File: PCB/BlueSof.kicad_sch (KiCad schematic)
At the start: 109 parts, among them J1 USB_C_Receptacle_USB2.0, J2 Conn_01x01_Female, J3 Conn_01x04_Female, J4 Conn_01x01_Female, J5 USB_C_Receptacle_USB2.0, Q1 A03407, Q2 A03407, SW1 SW_PUSH, SW10 SW_PUSH, SW11 SW_PUSH, SW12 SW_PUSH, SW13 SW_PUSH, SW14 SW_PUSH, SW15 SW_PUSH, SW16 SW_PUSH, SW17 SW_PUSH, SW18 SW_PUSH, SW19 SW_PUSH, SW2 SW_PUSH, SW20 SW_PUSH, SW21 SW_PUSH, SW22 SW_PUSH, SW23 SW_PUSH, SW24 SW_PUSH, SW25 Rotary_Encoder_Switch, SW26 SW_PUSH, SW27 SW_PUSH, SW28 SW_PUSH, SW29 SW_PUSH, SW3 SW_PUSH, SW30 SW_PUSH, SW31 SW_Push, SW32 SW_Push, SW4 SW_PUSH, SW5 SW_PUSH, SW6 SW_PUSH, SW7 SW_PUSH, SW8 SW_PUSH, SW9 SW_PUSH, U1 LN2054Y42AMR, U2 E73-2G4M08S1C, U3 AP2112K-3.3, U4 E73-2G4M08S1C, U5 LN2054Y42AMR, U6 AP2112K-3.3, Y1 32.768kHz, Y2 32.768kHz

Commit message: first commit, side 1
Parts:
- removed C10: 10uF, Capacitor_SMD:C_0603_1608Metric_Pad1.08x0.95mm_HandSolder, symbol Device:C_Small
- removed C6, C7: 22pF, Capacitor_SMD:C_0603_1608Metric_Pad1.08x0.95mm_HandSolder, symbol Device:C_Small
- removed C8, C9: 4.7uF, Capacitor_SMD:C_0603_1608Metric_Pad1.08x0.95mm_HandSolder, symbol Device:C_Small
- removed D29, D30: D, BlueSof:Diode_SOD123, symbol BlueSof-rescue:D-Lily58-cache-Lily58_Pro-rescue-SofleKeyboard-rescue
- removed D34, D36: LED, LED_SMD:LED_0603_1608Metric_Pad1.05x0.95mm_HandSolder, symbol Device:LED
- removed D35: 1N5819, Diode_SMD:D_SOD-323_HandSoldering, symbol Diode:1N5819
- removed J5: USB_C_Receptacle_USB2.0, Connector_USB:USB_C_Receptacle_HRO_TYPE-C-31-M-12, symbol Connector:USB_C_Receptacle_USB2.0
- removed Q1: A03407, Package_TO_SOT_SMD:SOT-23, symbol Device:Q_PMOS_GSD
- removed R10: 2M, Resistor_SMD:R_0603_1608Metric_Pad0.98x0.95mm_HandSolder, symbol Device:R_Small
- removed R11, R15: 1k, Resistor_SMD:R_0603_1608Metric_Pad0.98x0.95mm_HandSolder, symbol Device:R_Small
- removed R12, R13: 5.1k, Resistor_SMD:R_0603_1608Metric_Pad0.98x0.95mm_HandSolder, symbol Device:R_Small
- removed R14: 100k, Resistor_SMD:R_0603_1608Metric_Pad0.98x0.95mm_HandSolder, symbol Device:R_Small
- removed R16: 10k, Resistor_SMD:R_0603_1608Metric_Pad0.98x0.95mm_HandSolder, symbol Device:R_Small
- removed R3: 820k, Resistor_SMD:R_0603_1608Metric_Pad0.98x0.95mm_HandSolder, symbol Device:R_Small
- removed SW29, SW30: SW_PUSH, BlueSof:KailhLowProfile, symbol BlueSof-rescue:SW_PUSH-Lily58-cache-Lily58_Pro-rescue-SofleKeyboard-rescue
- removed SW32: SW_Push, Button_Switch_SMD:SW_SPST_B3U-1000P, symbol Switch:SW_Push
- removed U4: E73-2G4M08S1C, BlueSof:E73-2G4M08S1C-52840, symbol BlueSof-rescue:E73-2G4M08S1C-ELLOW
- removed U5: LN2054Y42AMR, Package_TO_SOT_SMD:SOT-23-5, symbol BlueSof-rescue:LN2054Y42AMR-ELLOW
- removed U6: AP2112K-3.3, Package_TO_SOT_SMD:SOT-23-5, symbol Regulator_Linear:AP2112K-3.3
- removed Y2: 32.768kHz, Crystal:Crystal_SMD_MicroCrystal_CM9V-T1A-2Pin_1.6x1.0mm_HandSoldering, symbol Device:Crystal
- added J9: Conn_01x04_Female, Connector_PinHeader_2.54mm:PinHeader_1x04_P2.54mm_Vertical, symbol Connector:Conn_01x04_Female
- added SW59: SW_SPDT, Button_Switch_THT:SW_CuK_OS102011MA1QN1_SPDT_Angled, symbol Switch:SW_SPDT
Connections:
- net DATA+: now also J9.3 (Pin_3)
- net DATA-: now also J9.4 (Pin_4)
- net ENCA: now also U2.33 (P0.13); no longer U2.10 (P0.30/AIN6)
- net ENCB: now also U2.35 (P0.24); no longer U2.9 (P0.31/AIN7)
- net GND: now also J9.1 (Pin_1)
- net VBAT: now also SW59.1 (A); no longer Q2.3 (D)
- net VBUS: now also J9.2 (Pin_2)
- net row1: now also U2.10 (P0.30/AIN6); no longer U2.33 (P0.13)
- net row2: now also U2.9 (P0.31/AIN7); no longer U2.35 (P0.24)
- new net: Q2.3 (D), SW59.2 (B)
- no-connect marks 32 -> 16
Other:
- note added: "USB Header"
- note removed: "Left Side"
- moved on the sheet: C1, C2, C3, C4, C5, D1, D10, D11, D12, D13, D14, D15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

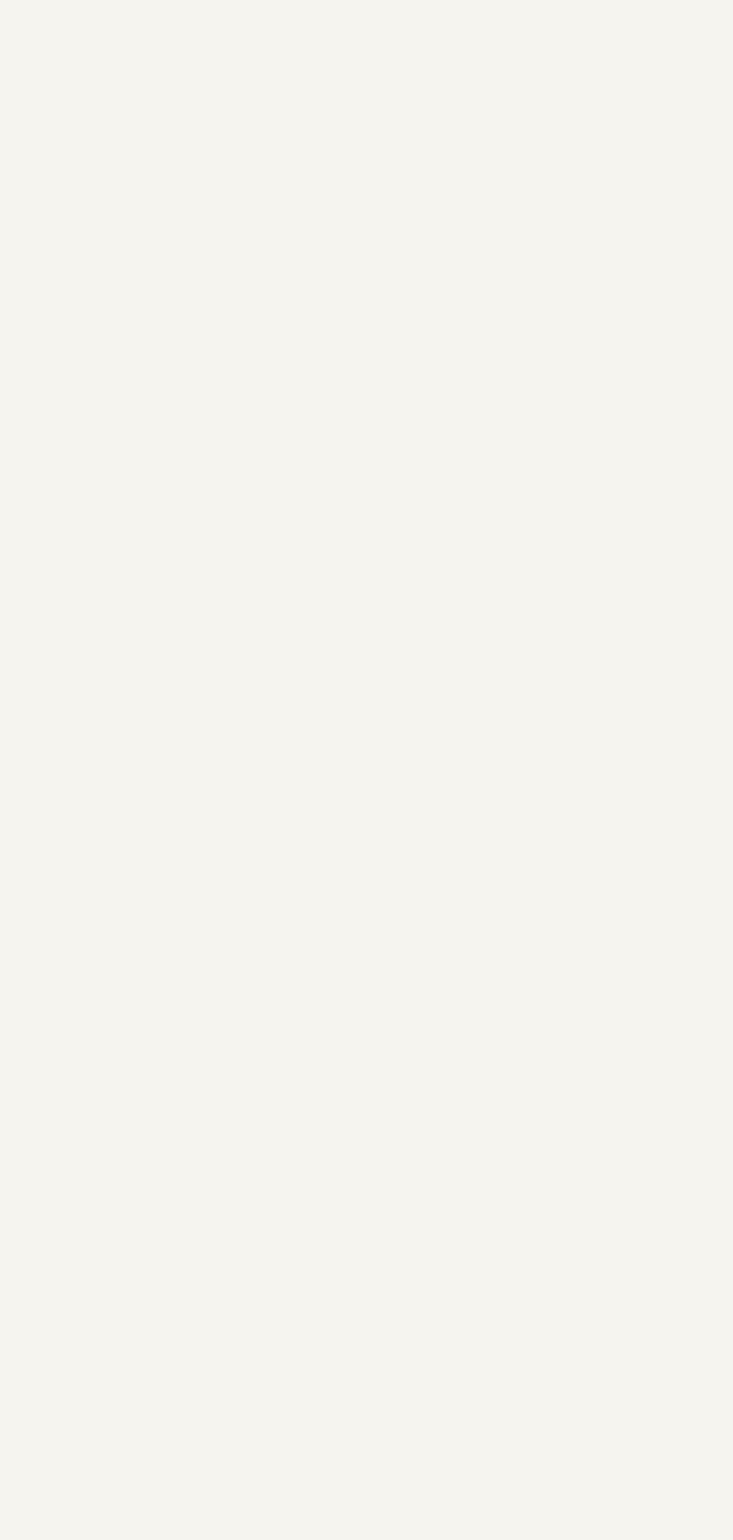
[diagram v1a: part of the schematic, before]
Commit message: EOD
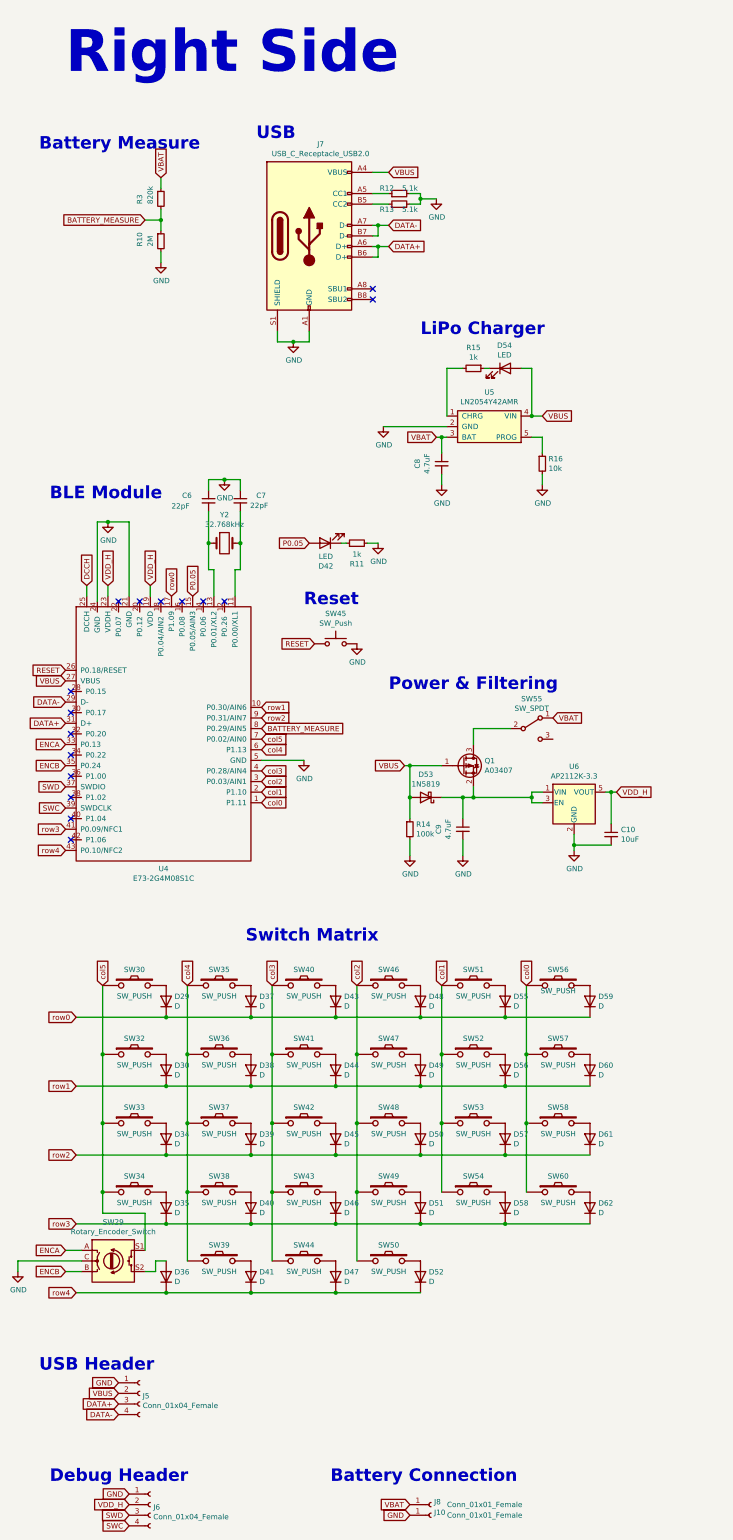
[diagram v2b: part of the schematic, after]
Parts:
- added C10: 10uF, Capacitor_SMD:C_0603_1608Metric_Pad1.08x0.95mm_HandSolder, symbol Device:C_Small
- added C6, C7: 22pF, Capacitor_SMD:C_0603_1608Metric_Pad1.08x0.95mm_HandSolder, symbol Device:C_Small
- added C8, C9: 4.7uF, Capacitor_SMD:C_0603_1608Metric_Pad1.08x0.95mm_HandSolder, symbol Device:C_Small
- added D29, D30, D34, D35, D36, D37, D38, D39, D40, D41, D43, D44, D45, D46, D47, D48, D49, D50, D51, D52, D55, D56, D57, D58, D59, D60, D61, D62: D, BlueSof:Diode_SOD123, symbol BlueSof-rescue:D-Lily58-cache-Lily58_Pro-rescue-SofleKeyboard-rescue
- added D42, D54: LED, LED_SMD:LED_0603_1608Metric_Pad1.05x0.95mm_HandSolder, symbol Device:LED
- added D53: 1N5819, Diode_SMD:D_SOD-323_HandSoldering, symbol Diode:1N5819
- added J10, J8: Conn_01x01_Female, Connector_PinHeader_2.54mm:PinHeader_1x01_P2.54mm_Vertical, symbol Connector:Conn_01x01_Female
- added J5, J6: Conn_01x04_Female, Connector_PinHeader_2.54mm:PinHeader_1x04_P2.54mm_Vertical, symbol Connector:Conn_01x04_Female
- added J7: USB_C_Receptacle_USB2.0, BlueSof:USB-C_C168688, symbol Connector:USB_C_Receptacle_USB2.0
- added Q1: A03407, Package_TO_SOT_SMD:SOT-23, symbol Device:Q_PMOS_GSD
- added R10: 2M, Resistor_SMD:R_0603_1608Metric_Pad0.98x0.95mm_HandSolder, symbol Device:R_Small
- added R11, R15: 1k, Resistor_SMD:R_0603_1608Metric_Pad0.98x0.95mm_HandSolder, symbol Device:R_Small
- added R12, R13: 5.1k, Resistor_SMD:R_0603_1608Metric_Pad0.98x0.95mm_HandSolder, symbol Device:R_Small
- added R14: 100k, Resistor_SMD:R_0603_1608Metric_Pad0.98x0.95mm_HandSolder, symbol Device:R_Small
- added R16: 10k, Resistor_SMD:R_0603_1608Metric_Pad0.98x0.95mm_HandSolder, symbol Device:R_Small
- added R3: 820k, Resistor_SMD:R_0603_1608Metric_Pad0.98x0.95mm_HandSolder, symbol Device:R_Small
- added SW29: Rotary_Encoder_Switch, Rotary_Encoder:RotaryEncoder_Alps_EC11E-Switch_Vertical_H20mm, symbol BlueSof-rescue:Rotary_Encoder_Switch-Device-SofleKeyboard-rescue
- added SW30, SW32, SW33, SW34, SW35, SW36, SW37, SW38, SW40, SW41, SW42, SW43, SW44, SW46, SW47, SW48, SW49, SW50, SW51, SW52, SW53, SW54, SW56, SW57, SW58, SW60: SW_PUSH, BlueSof:KailhLowProfile, symbol BlueSof-rescue:SW_PUSH-Lily58-cache-Lily58_Pro-rescue-SofleKeyboard-rescue
- added SW39: SW_PUSH, BlueSof:KailhLowProfile_1.5U, symbol BlueSof-rescue:SW_PUSH-Lily58-cache-Lily58_Pro-rescue-SofleKeyboard-rescue
- added SW45: SW_Push, Button_Switch_SMD:SW_SPST_B3U-1000P, symbol Switch:SW_Push
- added SW55: SW_SPDT, Button_Switch_THT:SW_CuK_OS102011MA1QN1_SPDT_Angled, symbol Switch:SW_SPDT
- added U4: E73-2G4M08S1C, BlueSof:E73-2G4M08S1C-52840, symbol BlueSof-rescue:E73-2G4M08S1C-ELLOW
- added U5: LN2054Y42AMR, Package_TO_SOT_SMD:SOT-23-5, symbol BlueSof-rescue:LN2054Y42AMR-ELLOW
- added U6: AP2112K-3.3, Package_TO_SOT_SMD:SOT-23-5, symbol Regulator_Linear:AP2112K-3.3
- added Y2: 32.768kHz, Crystal:Crystal_SMD_MicroCrystal_CM9V-T1A-2Pin_1.6x1.0mm_HandSoldering, symbol Device:Crystal
- J1: footprint Connector_USB:USB_C_Receptacle_HRO_TYPE-C-31-M-12 -> BlueSof:USB-C_C168688
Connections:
- net BATTERY_MEASURE: now also R10.1, R3.2, U4.8 (P0.29/AIN5)
- net DATA+: now also J5.3 (Pin_3), J7.A6 (D+), J7.B6 (D+), U4.31 (D+)
- net DATA-: now also J5.4 (Pin_4), J7.A7 (D-), J7.B7 (D-), U4.29 (D-)
- net DCCH: now also U4.25 (DCCH)
- net ENCA: now also SW29.A, U4.33 (P0.13)
- net ENCB: now also SW29.B, U4.35 (P0.24)
- net GND: now also C10.2, C6.1, C7.1, C8.2, C9.2, J10.1 (Pin_1), J5.1 (Pin_1), J6.1 (Pin_1), J7.A1 (GND), J7.A12 (GND), J7.B1 (GND), J7.B12 (GND), J7.S1 (SHIELD), R10.2, R11.2, R12.2, R13.2, R14.2, R16.2, SW29.C, SW45.2, U4.21 (GND), U4.24 (GND), U4.5 (GND), U5.2 (GND), U6.2 (GND)
- net P0.05: now also D42.2 (A), U4.15 (P0.05/AIN3)
- net RESET: now also SW45.1, U4.26 (P0.18/RESET)
- net SWC: now also J6.4 (Pin_4), U4.39 (SWDCLK)
- net SWD: now also J6.3 (Pin_3), U4.37 (SWDIO)
- net VBAT: now also C8.1, J8.1 (Pin_1), R3.1, SW55.1 (A), U5.3 (BAT)
- net VBUS: now also D53.2 (A), D54.2 (A), J5.2 (Pin_2), J7.A4 (VBUS), J7.A9 (VBUS), J7.B4 (VBUS), J7.B9 (VBUS), Q1.1 (G), R14.1, U4.27 (VBUS), U5.4 (VIN)
- net VDD_H: now also C10.1, J6.2 (Pin_2), U4.19 (VDD), U4.23 (VDDH), U6.5 (VOUT)
- net col0: now also SW56.1, SW57.1, SW58.1, SW60.1, U4.1 (P1.11)
- net col1: now also SW51.1, SW52.1, SW53.1, SW54.1, U4.2 (P1.10)
- net col2: now also SW46.1, SW47.1, SW48.1, SW49.1, SW50.1, U4.3 (P0.03/AIN1)
- net col3: now also SW40.1, SW41.1, SW42.1, SW43.1, SW44.1, U4.4 (P0.28/AIN4)
- net col4: now also SW35.1, SW36.1, SW37.1, SW38.1, SW39.1, U4.6 (P1.13)
- net col5: now also SW29.S1, SW30.1, SW32.1, SW33.1, SW34.1, U4.7 (P0.02/AIN0)
- net row0: now also D29.1 (K), D37.1 (K), D43.1 (K), D48.1 (K), D55.1 (K), D59.1 (K), U4.17 (P1.09)
- net row1: now also D30.1 (K), D38.1 (K), D44.1 (K), D49.1 (K), D56.1 (K), D60.1 (K), U4.10 (P0.30/AIN6)
- net row2: now also D34.1 (K), D39.1 (K), D45.1 (K), D50.1 (K), D57.1 (K), D61.1 (K), U4.9 (P0.31/AIN7)
- net row3: now also D35.1 (K), D40.1 (K), D46.1 (K), D51.1 (K), D58.1 (K), D62.1 (K), U4.41 (P0.09/NFC1)
- net row4: now also D36.1 (K), D41.1 (K), D47.1 (K), D52.1 (K), U4.43 (P0.10/NFC2)
- new net: J7.A5 (CC1), R12.1
- new net: J7.B5 (CC2), R13.1
- new net: D54.1 (K), R15.1
- new net: R15.2, U5.1 (CHRG)
- new net: D60.2 (A), SW57.2
- new net: D40.2 (A), SW38.2
- new net: D52.2 (A), SW50.2
- new net: D62.2 (A), SW60.2
- new net: C7.2, U4.11 (P0.00/XL1), Y2.2
- new net: C6.2, U4.13 (P0.01/XL2), Y2.1
- new net: D44.2 (A), SW41.2
- new net: D56.2 (A), SW52.2
- new net: D29.2 (A), SW30.2
- new net: D39.2 (A), SW37.2
- new net: D46.2 (A), SW43.2
- new net: Q1.3 (D), SW55.2 (B)
- new net: D34.2 (A), SW33.2
- new net: D48.2 (A), SW46.2
- new net: D49.2 (A), SW47.2
- new net: D37.2 (A), SW35.2
- new net: D61.2 (A), SW58.2
- new net: D30.2 (A), SW32.2
- new net: D45.2 (A), SW42.2
- new net: D41.2 (A), SW39.2
- new net: D36.2 (A), SW29.S2
- new net: D47.2 (A), SW44.2
- new net: D57.2 (A), SW53.2
- new net: C9.1, D53.1 (K), Q1.2 (S), U6.1 (VIN), U6.3 (EN)
- new net: D55.2 (A), SW51.2
- new net: D59.2 (A), SW56.2
- new net: D35.2 (A), SW34.2
- new net: R16.1, U5.5 (PROG)
- new net: D51.2 (A), SW49.2
- new net: D42.1 (K), R11.1
- new net: D50.2 (A), SW48.2
- new net: D43.2 (A), SW40.2
- new net: D58.2 (A), SW54.2
- new net: D38.2 (A), SW36.2
- no-connect marks 16 -> 32

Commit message: getting close to layout on side 1
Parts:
- D1, D10, D11, D12, D13, D14, D15, D16, D17, D18, D19, D2, D20, D21, D22, D23, D24, D25, D26, D27, D28, D29, D3, D30, D34, D35, D36, D37, D38, D39, D4, D40, D41, D43, D44, D45, D46, D47, D48, D49, D5, D50, D51, D52, D55, D56, D57, D58, D59, D6, D60, D61, D62, D7, D8, D9: footprint BlueSof:Diode_SOD123 -> Diode_SMD:D_SOD-123; symbol BlueSof-rescue:D-Lily58-cache-Lily58_Pro-rescue-SofleKeyboard-rescue -> Diode:1N4148
- SW1, SW10, SW11, SW12, SW13, SW14, SW15, SW16, SW17, SW18, SW19, SW2, SW20, SW21, SW22, SW23, SW24, SW26, SW27, SW28, SW3, SW30, SW32, SW33, SW34, SW35, SW36, SW37, SW38, SW39, SW4, SW40, SW41, SW42, SW43, SW44, SW46, SW47, SW48, SW49, SW5, SW50, SW51, SW52, SW53, SW54, SW56, SW57, SW58, SW6, SW60, SW7, SW8, SW9: symbol BlueSof-rescue:SW_PUSH-Lily58-cache-Lily58_Pro-rescue-SofleKeyboard-rescue -> Switch:SW_Push
- U2, U4: symbol BlueSof-rescue:E73-2G4M08S1C-ELLOW -> BlueSof:E73-2G4M08S1C
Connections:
- net BATTERY_MEASURE: no longer R10.1, R3.2, U4.8 (P0.29/AIN5)
- net DATA+: no longer J5.3 (Pin_3), J7.A6 (D+), J7.B6 (D+), U4.31 (D+)
- net DATA-: no longer J5.4 (Pin_4), J7.A7 (D-), J7.B7 (D-), U4.29 (D-)
- net DCCH: no longer U4.25 (DCCH)
- net ENCA: no longer SW29.A, U4.33 (P0.13)
- net ENCB: no longer SW29.B, U4.35 (P0.24)
- net GND: no longer C10.2, C6.1, C7.1, C8.2, C9.2, J10.1 (Pin_1), J5.1 (Pin_1), J6.1 (Pin_1), J7.A1 (GND), J7.A12 (GND), J7.B1 (GND), J7.B12 (GND), J7.S1 (SHIELD), R10.2, R11.2, R14.2, R16.2, SW29.C, SW45.2, U4.21 (GND), U4.24 (GND), U4.5 (GND), U5.2 (GND), U6.2 (GND)
- net P0.05: no longer D42.2 (A), U4.15 (P0.05/AIN3)
- net RESET: no longer SW45.1, U4.26 (P0.18/RESET)
- net SWC: no longer J6.4 (Pin_4), U4.39 (SWDCLK)
- net SWD: no longer J6.3 (Pin_3), U4.37 (SWDIO)
- net VBAT: no longer C8.1, J8.1 (Pin_1), R3.1, SW55.1 (A), U5.3 (BAT)
- net VBUS: no longer D53.2 (A), D54.2 (A), J5.2 (Pin_2), J7.A4 (VBUS), J7.A9 (VBUS), J7.B4 (VBUS), J7.B9 (VBUS), Q1.1 (G), R14.1, U4.27 (VBUS), U5.4 (VIN)
- net VDD_H: no longer C10.1, J6.2 (Pin_2), U4.19 (VDD), U4.23 (VDDH), U6.5 (VOUT)
- net col0: now also D23.2 (A), D5.2 (A), SW23.2, SW5.2; no longer SW12.1, SW18.1, SW56.1, SW57.1, SW58.1, SW60.1, U4.1 (P1.11)
- net col1: now also D22.2 (A), D4.2 (A), SW22.2, SW4.2; no longer SW11.1, SW17.1, SW51.1, SW52.1, SW53.1, SW54.1, U4.2 (P1.10)
- net col2: now also D27.2 (A), D3.2 (A), SW27.2, SW3.2; no longer SW10.1, SW16.1, SW22.1, SW46.1, SW47.1, SW48.1, SW49.1, SW50.1, U4.3 (P0.03/AIN1)
- net col3: now also D2.2 (A), D26.2 (A), SW2.2, SW26.2; no longer SW15.1, SW21.1, SW40.1, SW41.1, SW42.1, SW43.1, SW44.1, SW9.1, U4.4 (P0.28/AIN4)
- net col4: now also D1.2 (A), SW1.2; no longer SW14.1, SW20.1, SW35.1, SW36.1, SW37.1, SW38.1, SW39.1, SW8.1, U4.6 (P1.13)
- net col5: no longer SW29.S1, SW30.1, SW32.1, SW33.1, SW34.1, U4.7 (P0.02/AIN0)
- net row0: no longer D29.1 (K), D37.1 (K), D43.1 (K), D48.1 (K), D55.1 (K), D59.1 (K), U4.17 (P1.09)
- net row1: no longer D30.1 (K), D38.1 (K), D44.1 (K), D49.1 (K), D56.1 (K), D60.1 (K), U4.10 (P0.30/AIN6)
- net row2: no longer D34.1 (K), D39.1 (K), D45.1 (K), D50.1 (K), D57.1 (K), D61.1 (K), U4.9 (P0.31/AIN7)
- net row3: no longer D35.1 (K), D40.1 (K), D46.1 (K), D51.1 (K), D58.1 (K), D62.1 (K), U4.41 (P0.09/NFC1)
- net row4: no longer D36.1 (K), D41.1 (K), D47.1 (K), D52.1 (K), U4.43 (P0.10/NFC2)
- net at D8.2 (A), SW8.2: now also SW9.1
- net at D9.2 (A), SW9.2: now also SW10.1
- net at D10.2 (A), SW10.2: now also SW11.1
- net at D11.2 (A), SW11.2: now also SW12.1
- net at D7.2 (A), SW7.2: now also SW8.1
- net at D13.2 (A), SW13.2: now also SW14.1
- net at D14.2 (A), SW14.2: now also SW15.1
- net at D15.2 (A), SW15.2: now also SW16.1
- net at D16.2 (A), SW16.2: now also SW17.1
- net at D17.2 (A), SW17.2: now also SW18.1
- net at D21.2 (A), SW21.2: now also SW22.1
- net at D20.2 (A), SW20.2: now also SW21.1
- net at D19.2 (A), SW19.2: now also SW20.1
- net at SW28.2: no longer D28.2 (A)
- net at D40.2 (A), SW38.2: now also SW43.1
- net at D44.2 (A), SW41.2: now also SW47.1
- net at D56.2 (A), SW52.2: now also SW57.1
- net col4_LEFT: now reaches D29.2 (A), SW30.2
- net col4_LEFT: now also SW35.1, SW39.1, U4.6 (P1.13)
- net at D39.2 (A), SW37.2: now also SW42.1
- net at D46.2 (A), SW43.2: now also SW49.1
- net at D34.2 (A), SW33.2: now also SW37.1
- net col1_LEFT: now reaches D48.2 (A), SW46.2
- net col1_LEFT: now also D51.2 (A), SW49.2, SW51.1, SW54.1, U4.2 (P1.10)
- net at D49.2 (A): now also SW52.1; no longer SW47.2
- net col3_LEFT: now reaches D37.2 (A), SW35.2
- net col3_LEFT: now also D41.2 (A), SW39.2, SW40.1, SW44.1, U4.4 (P0.28/AIN4)
- net at D30.2 (A), SW32.2: now also SW36.1
- net at D45.2 (A), SW42.2: now also SW48.1
- net col2_LEFT: now reaches D47.2 (A), SW44.2
- net col2_LEFT: now also D43.2 (A), SW40.2, SW46.1, SW50.1, U4.3 (P0.03/AIN1)
- net at D57.2 (A), SW53.2: now also SW58.1
- net col0_LEFT: now reaches D55.2 (A), SW51.2
- net col0_LEFT: now also D58.2 (A), SW54.2, SW56.1, SW60.1, U4.1 (P1.11)
- net at D35.2 (A), SW34.2: now also SW38.1
- net at D50.2 (A), SW48.2: now also SW53.1
- net at D38.2 (A), SW36.2: now also SW41.1
- new net BATTERY_MEASURE_LEFT: R10.1, R3.2, U4.8 (P0.29/AIN5)
- new net DATA+_LEFT: J5.3 (Pin_3), J7.A6 (D+), J7.B6 (D+), U4.31 (D+)
- new net DATA-_LEFT: J5.4 (Pin_4), J7.A7 (D-), J7.B7 (D-), U4.29 (D-)
- new net DCCH_LEFT: U4.25 (DCCH)
- new net ENCA_LEFT: SW29.A, U4.33 (P0.13)
- new net ENCB_LEFT: SW29.B, U4.35 (P0.24)
- new net GND2: C10.2, C6.1, C7.1, C8.2, C9.2, J10.1 (Pin_1), J5.1 (Pin_1), J6.1 (Pin_1), J7.A1 (GND), J7.A12 (GND), J7.B1 (GND), J7.B12 (GND), J7.S1 (SHIELD), R10.2, R11.2, R14.2, R16.2, SW29.C, SW45.2, U4.21 (GND), U4.24 (GND), U4.5 (GND), U5.2 (GND), U6.2 (GND)
- new net P0.05_LEFT: D42.2 (A), U4.15 (P0.05/AIN3)
- new net RESET_LEFT: SW45.1, U4.26 (P0.18/RESET)
- new net SWC_LEFT: J6.4 (Pin_4), U4.39 (SWDCLK)
- new net SWD_LEFT: J6.3 (Pin_3), U4.37 (SWDIO)
- new net VBAT_LEFT: C8.1, J8.1 (Pin_1), R3.1, SW55.1 (A), U5.3 (BAT)
- new net VBUS_LEFT: D53.2 (A), D54.2 (A), J5.2 (Pin_2), J7.A4 (VBUS), J7.A9 (VBUS), J7.B4 (VBUS), J7.B9 (VBUS), Q1.1 (G), R14.1, U4.27 (VBUS), U5.4 (VIN)
- new net VDD_H_LEFT: C10.1, J6.2 (Pin_2), U4.19 (VDD), U4.23 (VDDH), U6.5 (VOUT)
- new net col5_LEFT: SW29.S1, SW30.1, SW32.1, SW33.1, SW34.1, U4.7 (P0.02/AIN0)
- new net row0_LEFT: D29.1 (K), D37.1 (K), D43.1 (K), D48.1 (K), D55.1 (K), D59.1 (K), U4.17 (P1.09)
- new net row1_LEFT: D30.1 (K), D38.1 (K), D44.1 (K), D49.1 (K), D56.1 (K), D60.1 (K), U4.10 (P0.30/AIN6)
- new net row2_LEFT: D34.1 (K), D39.1 (K), D45.1 (K), D50.1 (K), D57.1 (K), D61.1 (K), U4.9 (P0.31/AIN7)
- new net row3_LEFT: D35.1 (K), D40.1 (K), D46.1 (K), D51.1 (K), D58.1 (K), D62.1 (K), U4.41 (P0.09/NFC1)
- new net row4_LEFT: D36.1 (K), D41.1 (K), D47.1 (K), D52.1 (K), U4.43 (P0.10/NFC2)
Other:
- note added: "Left Side"
- moved on the sheet: D1, D10, D11, D12, D13, D14, D15, D16, D17, D18, D19, D2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
